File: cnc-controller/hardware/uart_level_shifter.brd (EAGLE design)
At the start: 14 parts, among them CN1 1X4-3.5MM, CN2 1X4-3.5MM, IC1 MAX3222, J1 1X2-3.5MM, J2 1X2-3.5MM

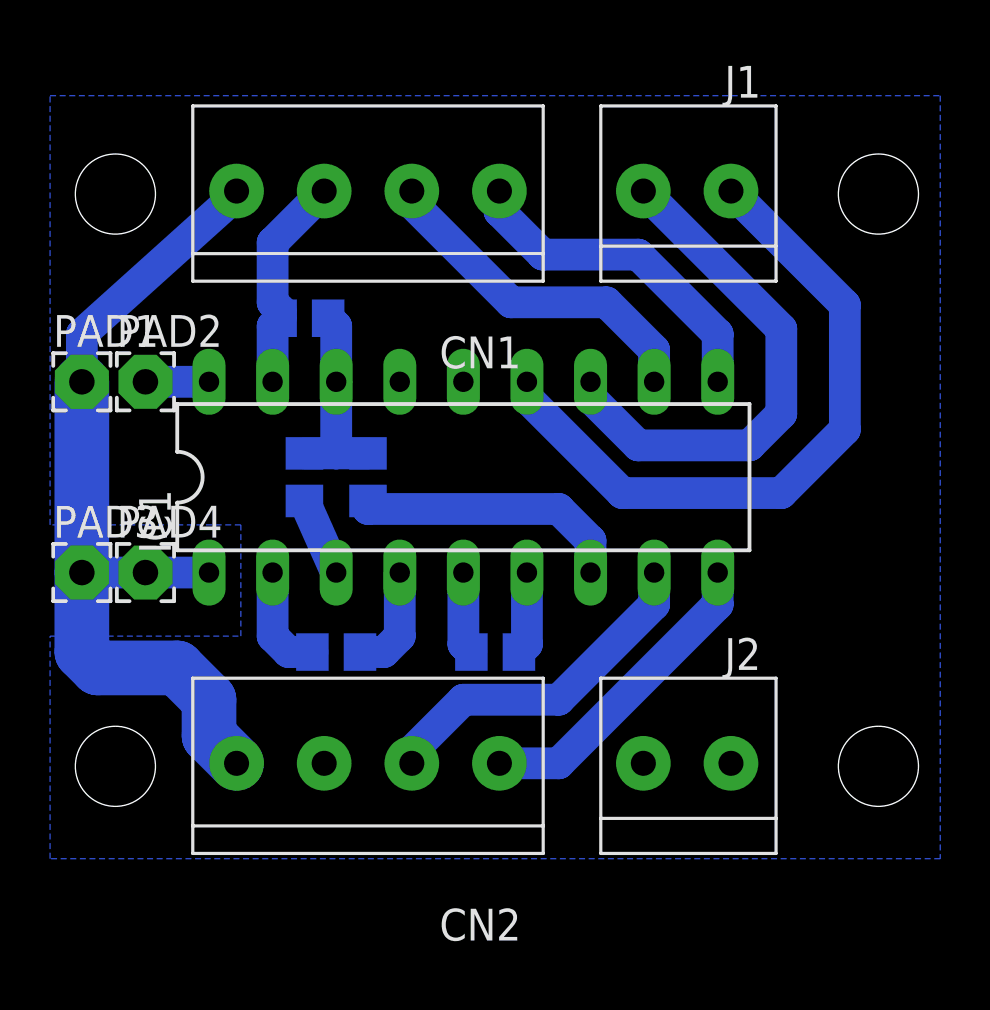
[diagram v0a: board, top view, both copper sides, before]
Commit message: cnc-controller mechanical
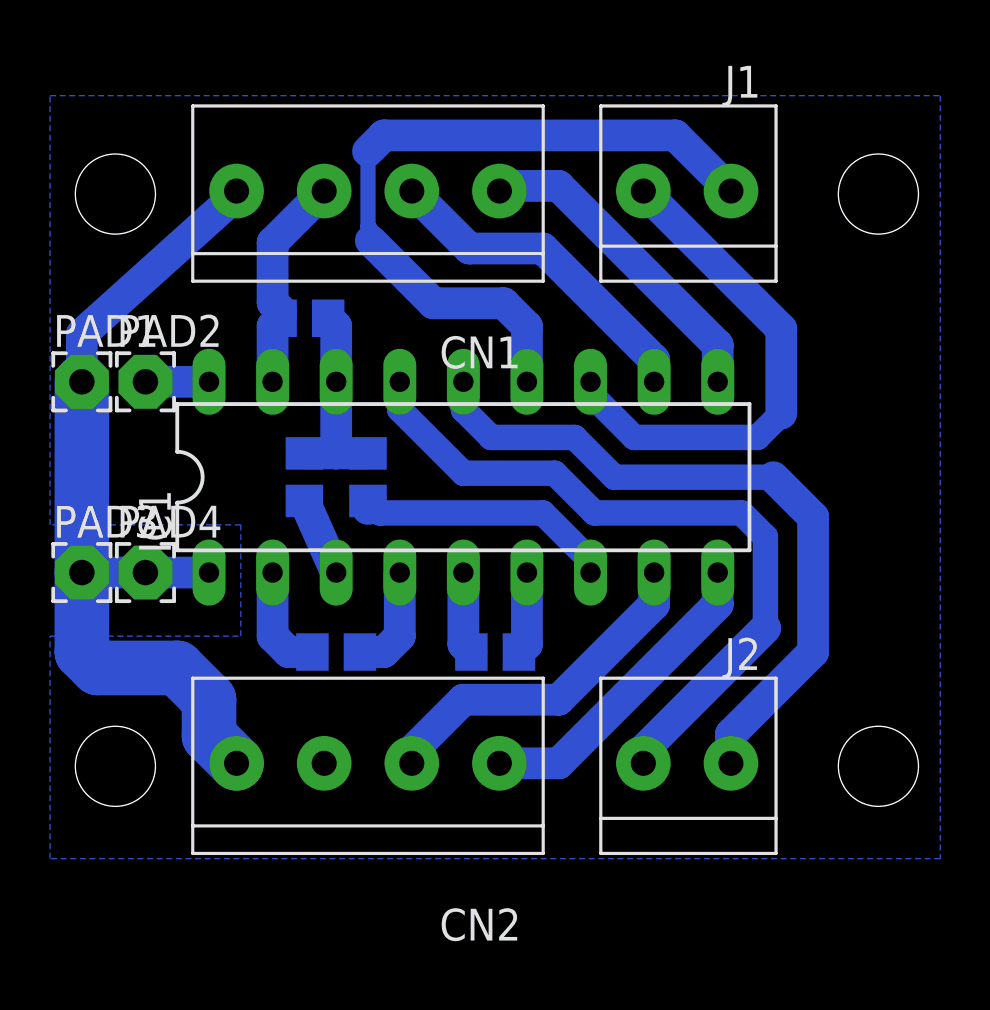
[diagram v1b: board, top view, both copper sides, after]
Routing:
- net T1OUT: track 0.00 -> 28.9 mm
- net R1IN: track 0.00 -> 28.1 mm
- net R1OUT: track 27.4 -> 29.2 mm
- net R2OUT: track 13.5 -> 12.9 mm
- net T2IN: track 13.9 -> 13.4 mm
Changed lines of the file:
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@@
 <setting verticaltext="up"/>
 </settings>
-<grid distance="2.54" unitdist="mm" unit="mm" style="lines" multiple="1" display="yes" altdistance="0.635" altunitdist="mm" altunit="mm"/>
+<grid distance="2.54" unitdist="mm" unit="mm" style="lines" multiple="1" display="yes" altdistance="6.25" altunitdist="mil" altunit="mil"/>
 <layers>
 <layer number="1" name="Top" color="4" fill="1" visible="yes" active="yes"/>
@@
 <contactref element="J1" pad="2"/>
 <wire x1="21.59" y1="19.05" x2="21.59" y2="18.415" width="1.27" layer="16"/>
-<wire x1="21.59" y1="18.415" x2="23.495" y2="16.51" width="1.27" layer="16"/>
-<wire x1="23.495" y1="16.51" x2="27.94" y2="16.51" width="1.27" layer="16"/>
-<wire x1="27.94" y1="16.51" x2="29.21" y2="17.78" width="1.27" layer="16"/>
 <wire x1="29.21" y1="17.78" x2="29.21" y2="21.16" width="1.27" layer="16"/>
 <wire x1="29.21" y1="21.16" x2="23.7" y2="26.67" width="1.27" layer="16"/>
+<wire x1="21.59" y1="18.415" x2="21.74875" y2="18.415" width="1.016" layer="16"/>
+<wire x1="21.74875" y1="18.415" x2="23.33625" y2="16.8275" width="1.016" layer="16"/>
+<wire x1="23.33625" y1="16.8275" x2="28.2575" y2="16.8275" width="1.016" layer="16"/>
+<wire x1="28.2575" y1="16.8275" x2="29.21" y2="17.78" width="1.016" layer="16"/>
 </signal>
 <signal name="T2IN">
 <contactref element="IC1" pad="11"/>
 <contactref element="CN1" pad="3"/>
-<wire x1="14.45" y1="26.67" x2="14.45" y2="26.19" width="1.27" layer="16"/>
-<wire x1="14.45" y1="26.19" x2="18.415" y2="22.225" width="1.27" layer="16"/>
-<wire x1="18.415" y1="22.225" x2="22.225" y2="22.225" width="1.27" layer="16"/>
-<wire x1="22.225" y1="22.225" x2="24.13" y2="20.32" width="1.27" layer="16"/>
-<wire x1="24.13" y1="20.32" x2="24.13" y2="19.05" width="1.27" layer="16"/>
+<wire x1="24.13" y1="19.05" x2="24.13" y2="19.9325" width="1.27" layer="16"/>
+<wire x1="24.13" y1="19.9325" x2="19.6875" y2="24.375" width="1.27" layer="16"/>
+<wire x1="19.6875" y1="24.375" x2="16.745" y2="24.375" width="1.27" layer="16"/>
+<wire x1="16.745" y1="24.375" x2="14.45" y2="26.67" width="1.27" layer="16"/>
 </signal>
 <signal name="R1OUT">
 <contactref element="IC1" pad="13"/>
 <contactref element="J1" pad="1"/>
-<wire x1="19.05" y1="19.05" x2="19.05" y2="18.415" width="1.27" layer="16"/>
-<wire x1="19.05" y1="18.415" x2="22.86" y2="14.605" width="1.27" layer="16"/>
-<wire x1="22.86" y1="14.605" x2="29.21" y2="14.605" width="1.27" layer="16"/>
-<wire x1="29.21" y1="14.605" x2="31.75" y2="17.145" width="1.27" layer="16"/>
-<wire x1="31.75" y1="17.145" x2="31.75" y2="22.12" width="1.27" layer="16"/>
-<wire x1="31.75" y1="22.12" x2="27.2" y2="26.67" width="1.27" layer="16"/>
+<wire x1="19.05" y1="19.05" x2="19.05" y2="21.2625" width="1.27" layer="16"/>
+<wire x1="19.05" y1="21.2625" x2="18.125" y2="22.1875" width="1.27" layer="16"/>
+<wire x1="18.125" y1="22.1875" x2="15.3125" y2="22.1875" width="1.27" layer="16"/>
+<wire x1="15.3125" y1="22.1875" x2="12.8125" y2="24.6875" width="1.27" layer="16"/>
+<wire x1="12.8125" y1="24.6875" x2="12.8125" y2="25.12875" width="0.6096" layer="16"/>
+<wire x1="12.8125" y1="25.12875" x2="12.7" y2="25.24125" width="0.6096" layer="16"/>
+<wire x1="12.7" y1="25.24125" x2="12.7" y2="28.2575" width="0.6096" layer="16"/>
+<wire x1="12.7" y1="28.2575" x2="13.335" y2="28.8925" width="1.27" layer="16"/>
+<wire x1="13.335" y1="28.8925" x2="24.9775" y2="28.8925" width="1.27" layer="16"/>
+<wire x1="24.9775" y1="28.8925" x2="27.2" y2="26.67" width="1.27" layer="16"/>
 </signal>
 <signal name="R2OUT">
 <contactref element="IC1" pad="10"/>
 <contactref element="CN1" pad="4"/>
-<wire x1="17.95" y1="26.67" x2="17.95" y2="25.865" width="1.27" layer="16"/>
-<wire x1="17.95" y1="25.865" x2="19.685" y2="24.13" width="1.27" layer="16"/>
-<wire x1="19.685" y1="24.13" x2="23.495" y2="24.13" width="1.27" layer="16"/>
-<wire x1="23.495" y1="24.13" x2="26.67" y2="20.955" width="1.27" layer="16"/>
-<wire x1="26.67" y1="20.955" x2="26.67" y2="19.05" width="1.27" layer="16"/>
+<wire x1="26.67" y1="19.05" x2="26.67" y2="20.5175" width="1.27" layer="16"/>
+<wire x1="26.67" y1="20.5175" x2="20.3125" y2="26.875" width="1.27" layer="16"/>
+<wire x1="20.3125" y1="26.875" x2="18.155" y2="26.875" width="1.27" layer="16"/>
+<wire x1="18.155" y1="26.875" x2="17.95" y2="26.67" width="1.27" layer="16"/>
 </signal>
 <signal name="T1OUT">
 <contactref element="IC1" pad="15"/>
 <contactref element="J2" pad="2"/>
-<wire x1="23.7" y1="3.81" x2="13.97" y2="19.05" width="0" layer="19" extent="1-1"/>
+<wire x1="23.7" y1="3.81" x2="23.7" y2="4.3325" width="1.27" layer="16"/>
+<wire x1="23.7" y1="4.3325" x2="28.575" y2="9.2075" width="1.27" layer="16"/>
+<wire x1="28.575" y1="9.2075" x2="28.575" y2="12.85875" width="1.016" layer="16"/>
+<wire x1="28.575" y1="12.85875" x2="27.6225" y2="13.81125" width="1.016" layer="16"/>
+<wire x1="27.6225" y1="13.81125" x2="21.74875" y2="13.81125" width="1.016" layer="16"/>
+<wire x1="13.97" y1="17.93875" x2="13.97" y2="19.05" width="1.016" layer="16"/>
+<wire x1="21.74875" y1="13.81125" x2="20.16125" y2="15.39875" width="1.016" layer="16"/>
+<wire x1="20.16125" y1="15.39875" x2="16.51" y2="15.39875" width="1.016" layer="16"/>
+<wire x1="16.51" y1="15.39875" x2="13.97" y2="17.93875" width="1.016" layer="16"/>
 </signal>
 <signal name="T2OUT">
@@
 <contactref element="IC1" pad="14"/>
 <contactref element="J2" pad="1"/>
-<wire x1="27.2" y1="3.81" x2="16.51" y2="19.05" width="0" layer="19" extent="1-1"/>
+<wire x1="27.2" y1="3.81" x2="27.2" y2="4.975" width="1.27" layer="16"/>
+<wire x1="27.2" y1="4.975" x2="30.48" y2="8.255" width="1.27" layer="16"/>
+<wire x1="30.48" y1="8.255" x2="30.48" y2="13.6525" width="1.27" layer="16"/>
+<wire x1="30.48" y1="13.6525" x2="28.8925" y2="15.24" width="1.27" layer="16"/>
+<wire x1="28.8925" y1="15.24" x2="22.5425" y2="15.24" width="1.016" layer="16"/>
+<wire x1="22.5425" y1="15.24" x2="20.955" y2="16.8275" width="1.016" layer="16"/>
+<wire x1="20.955" y1="16.8275" x2="17.62125" y2="16.8275" width="1.016" layer="16"/>
+<wire x1="17.62125" y1="16.8275" x2="16.51" y2="17.93875" width="1.016" layer="16"/>
+<wire x1="16.51" y1="17.93875" x2="16.51" y2="19.05" width="1.016" layer="16"/>
 </signal>
 <signal name="R2IN">
@@
 <contactref element="C4" pad="1"/>
 <wire x1="12.7" y1="14.29" x2="12.7" y2="13.97" width="1.27" layer="16"/>
-<wire x1="12.7" y1="13.97" x2="20.32" y2="13.97" width="1.27" layer="16"/>
-<wire x1="20.32" y1="13.97" x2="21.59" y2="12.7" width="1.27" layer="16"/>
-<wire x1="21.59" y1="12.7" x2="21.59" y2="11.43" width="1.27" layer="16"/>
+<wire x1="21.59" y1="11.43" x2="21.59" y2="11.90625" width="1.016" layer="16"/>
+<wire x1="21.59" y1="11.90625" x2="19.685" y2="13.81125" width="1.016" layer="16"/>
+<wire x1="19.685" y1="13.81125" x2="13.17875" y2="13.81125" width="1.016" layer="16"/>
+<wire x1="13.17875" y1="13.81125" x2="12.7" y2="14.29" width="1.016" layer="16"/>
 </signal>
 <signal name="N$9">
